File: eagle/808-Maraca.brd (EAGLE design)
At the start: 100 x 80 mm, 45 parts, among them IC1 TL071P, Q1 2N3904, Q2 2N3906, Q3 2N3906, Q4 2N3904, Q59 2N3904, Q60 2N3906

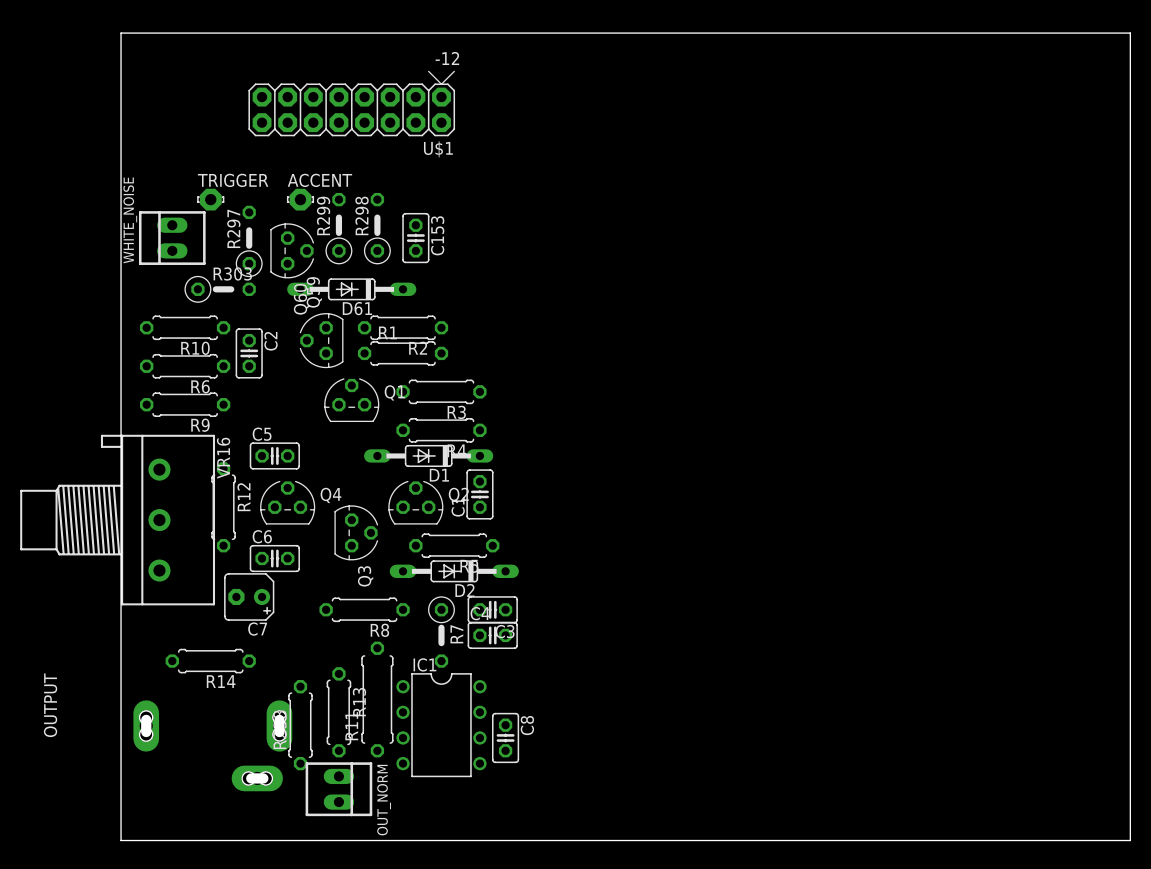
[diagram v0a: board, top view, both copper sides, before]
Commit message: well routed
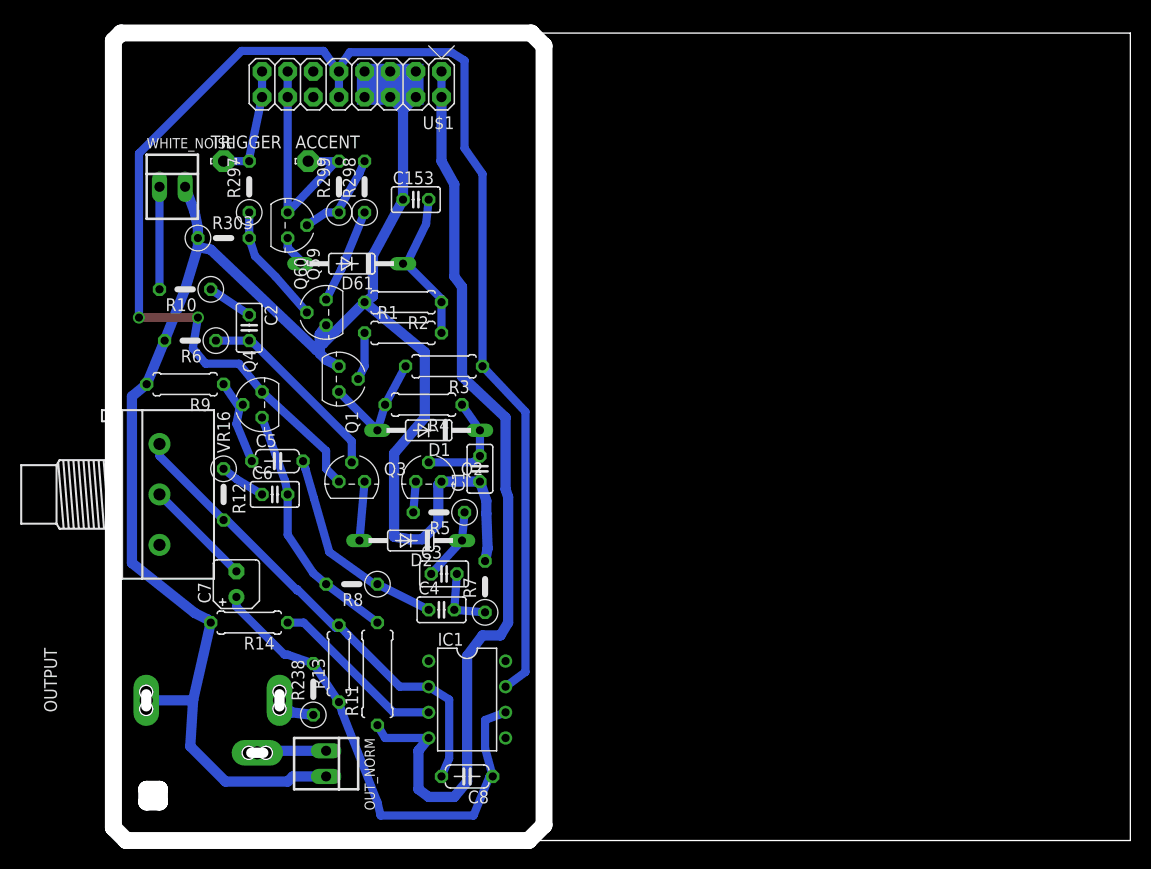
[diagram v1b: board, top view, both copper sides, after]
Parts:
- C5, C8: device TR808clone:C025-025X050 -> TR808clone:C050-024X044
- R10, R12, R238, R5, R6, R8: device TR808clone:0207/7 -> TR808clone:0207/5V
- moved Q4 10.5 mm to (14.0, 43.2), turned to 90 degrees
- moved R7 6.48 mm to (36.1, 25.1), turned to 90 degrees
- moved C6 6.35 mm to (15.2, 34.3)
- moved C3 5.99 mm to (32.0, 26.4), turned to 0 degrees
- moved C4 5.68 mm to (31.8, 22.9)
- moved C8 5.39 mm to (34.3, 6.35), turned to 180 degrees
- moved R14 5.39 mm to (12.7, 21.6)
- moved D2 5.29 mm to (28.7, 29.7)
- moved Q3 5.08 mm to (22.9, 35.6), turned to 0 degrees
- moved R297 5.08 mm to (12.7, 64.8)
- moved R303 5.08 mm to (10.2, 59.7)
- moved WHITE_NOISE 5.08 mm to (5.08, 64.8), turned to 0 degrees
- moved R13 4.83 mm to (21.6, 17.5), turned to 90 degrees
- moved TRIGGER 4.02 mm to (10.2, 67.3)
- moved R298 4.02 mm to (24.1, 64.8)
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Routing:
- net GND: track 0.00 -> 191.0 mm
- net +12V: track 0.00 -> 152.9 mm, vias 0 -> 2
- net -12V: track 0.00 -> 92.4 mm
- net N$8: track 0.00 -> 48.8 mm
- net N$17: track 0.00 -> 47.9 mm
- net N$16: track 0.00 -> 24.6 mm
- net TRIG: track 0.00 -> 24.0 mm
- net N$13: track 0.00 -> 20.8 mm
- net N$11: track 0.00 -> 20.0 mm
- net N$22: track 0.00 -> 17.7 mm
- net N$324: track 0.00 -> 15.5 mm
- net N$3: track 0.00 -> 12.4 mm
- net N$318: track 0.00 -> 12.0 mm
- net N$20: track 0.00 -> 11.6 mm
- net N$4: track 0.00 -> 11.0 mm
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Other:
- board size 100 x 80 mm -> 100.8 x 80 mm
